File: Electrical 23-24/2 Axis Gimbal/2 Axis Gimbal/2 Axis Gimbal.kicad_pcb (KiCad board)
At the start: 2 copper layers, 24.2 x 38.5 mm, 28 parts, among them IC1 BNO085, IC2 AP1086DL-13, J1 Conn_01x06_Socket, J2 Conn_01x06_Socket, U1 ATtiny404-SS

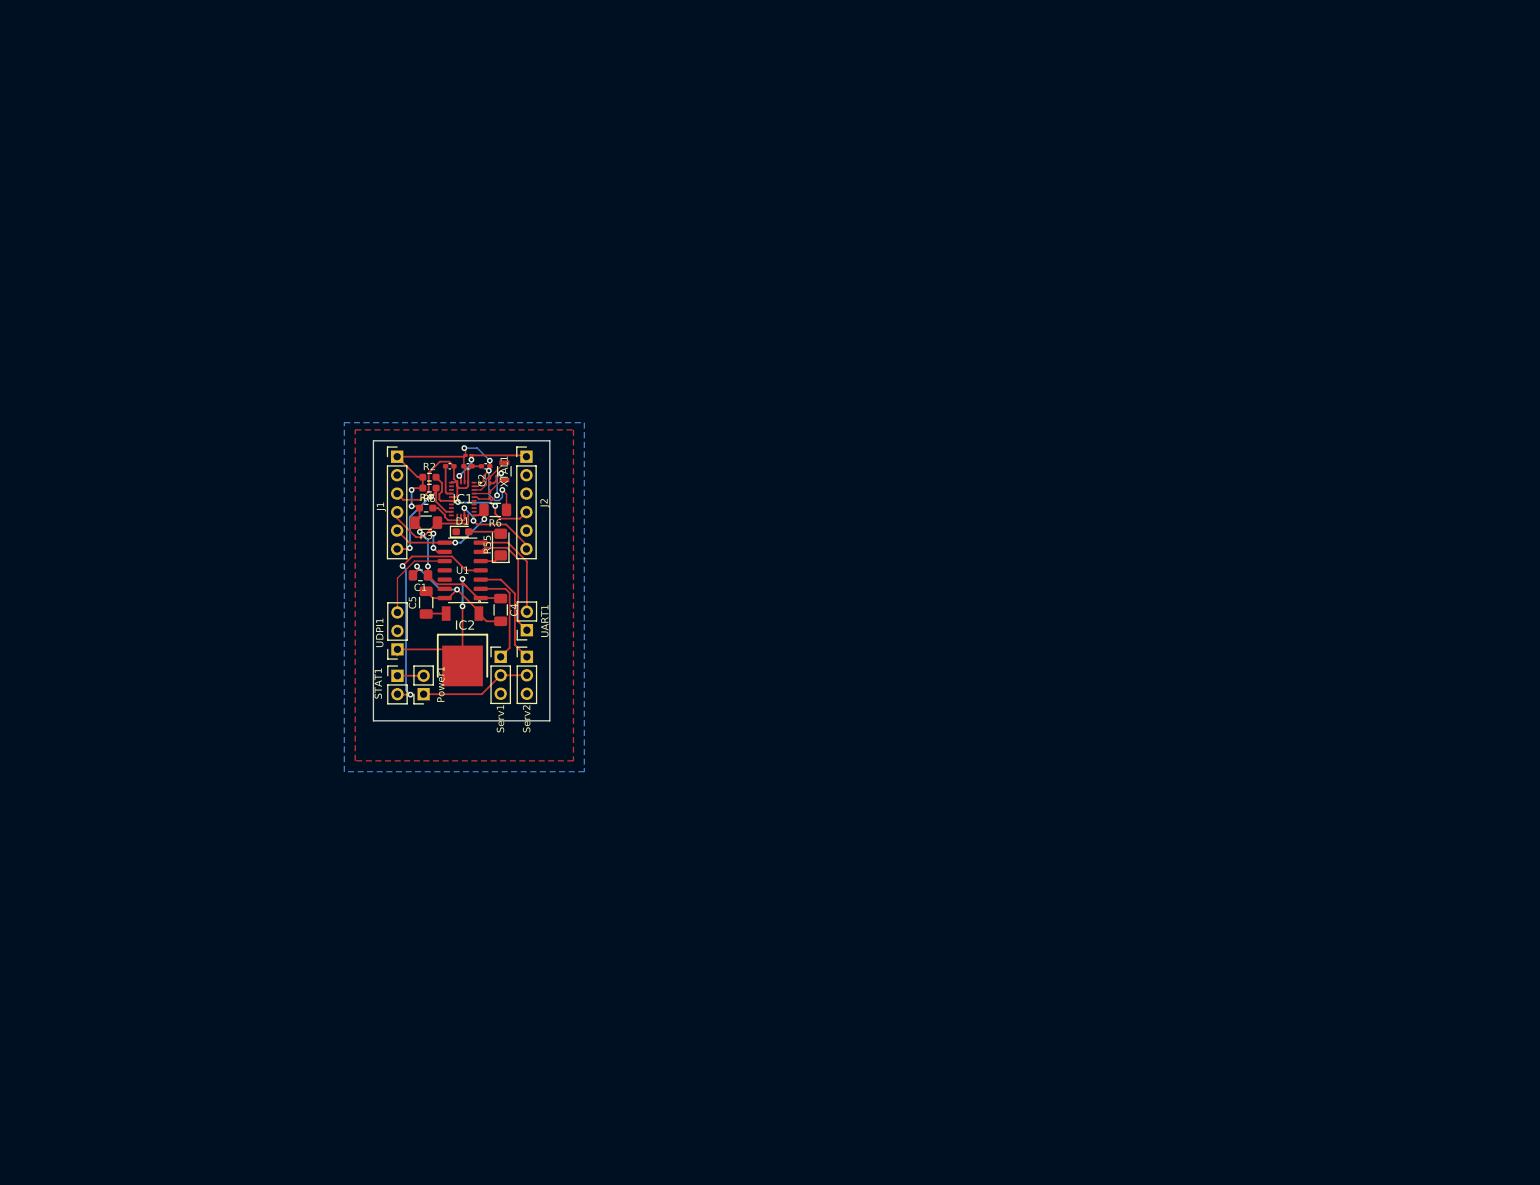
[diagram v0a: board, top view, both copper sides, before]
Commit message: Finished Gimbal Board
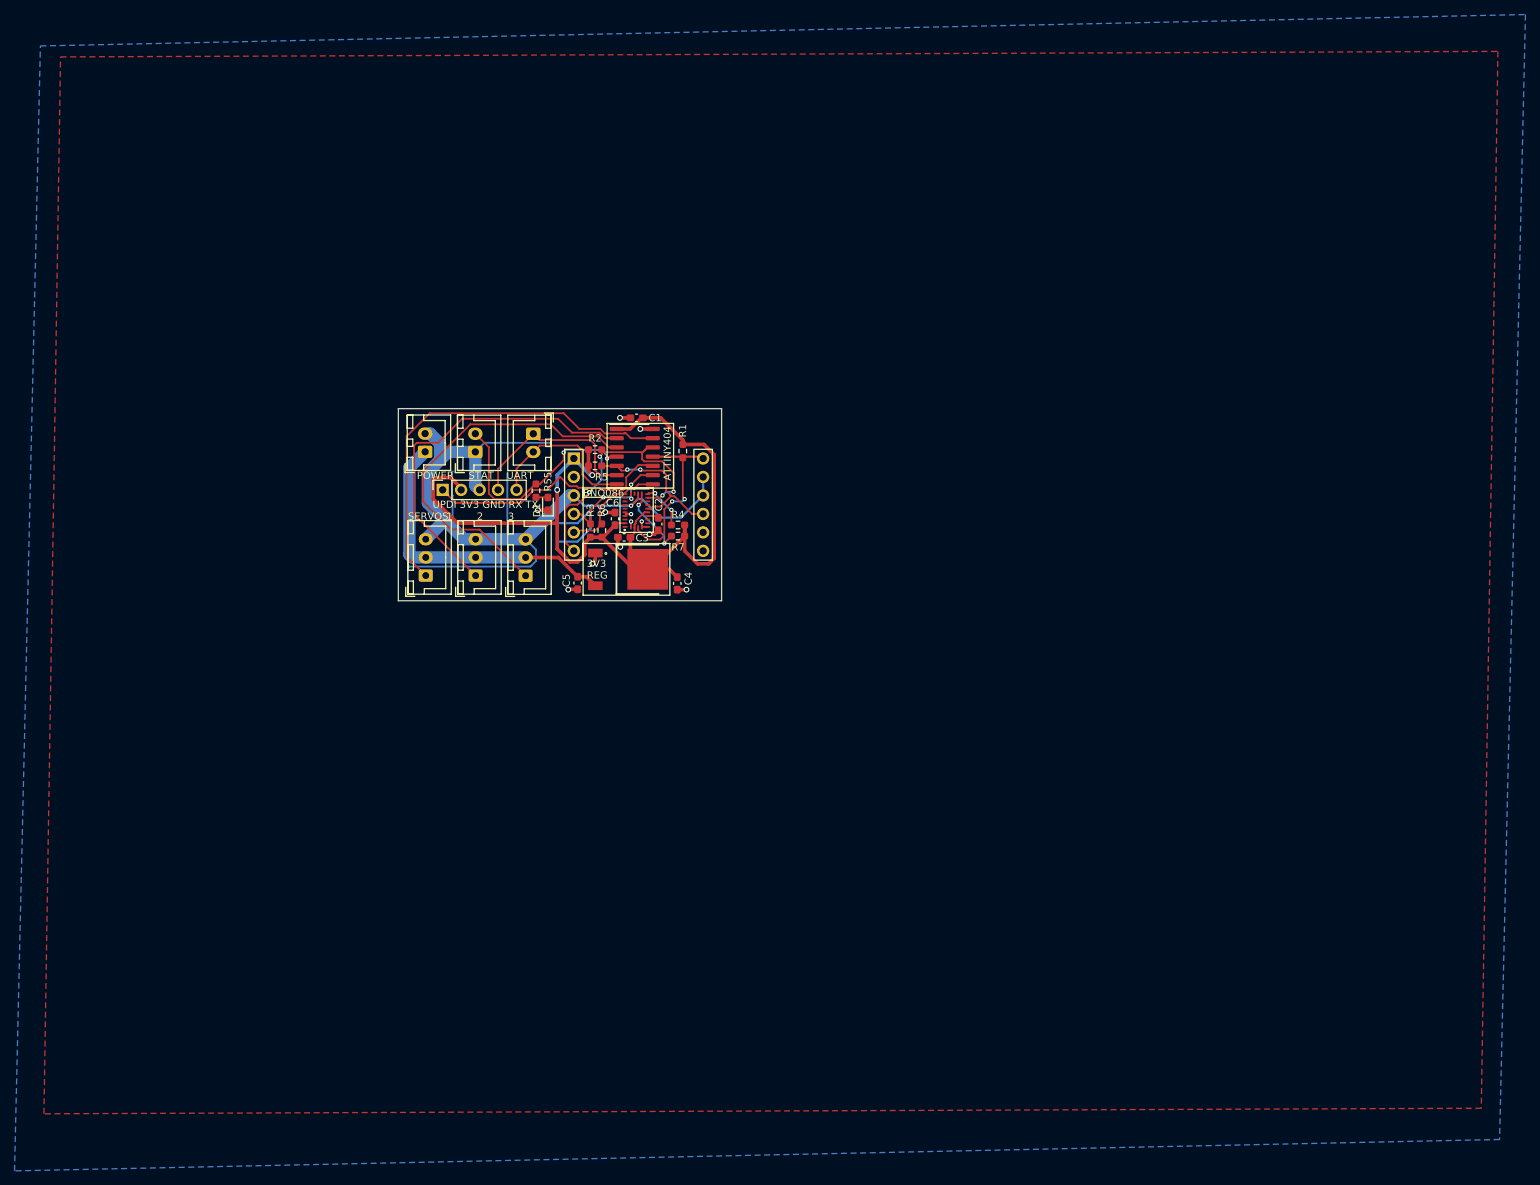
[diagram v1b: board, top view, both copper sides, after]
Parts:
- removed the C2 at (87.0, 77.9)
- removed the C3 at (87.0, 79.9)
- removed J1, J2: Conn_01x06_Socket, Connector_PinHeader_2.54mm:PinHeader_1x06_P2.54mm_Vertical
- removed XTAL1: ABS07-32.768KHZ-7-T, 32Crys:XTAL_ABS07-32.768KHZ-7-T_ABR
- added G***: LOGO, LOGO, B.Cu at (108.1, 81.3)
- added R7: 2.2k, Resistor_SMD:R_0603_1608Metric_Pad0.98x0.95mm_HandSolder, F.Cu at (112.9, 85.6)
- added Servo3: Conn_01x03_Pin, Connector_JST:JST_XH_B3B-XH-A_1x03_P2.50mm_Vertical, F.Cu at (91.9, 91.0)
- added U2: ~, gimbal:breakout, F.Cu at (107.4, 81.3)
- C1: value C_10uF -> 10u; footprint Capacitor_SMD:C_0805_2012Metric_Pad1.18x1.45mm_HandSolder -> Capacitor_SMD:C_0603_1608Metric_Pad1.08x0.95mm_HandSolder
- C2: renamed from D-CUP2; value C_0.1uF -> 0.1u; footprint Capacitor_SMD:C_0402_1005Metric_Pad0.74x0.62mm_HandSolder -> Capacitor_SMD:C_0603_1608Metric_Pad1.08x0.95mm_HandSolder
- C3: renamed from D-CUP3; value C_0.1uF -> 0.1u; footprint Capacitor_SMD:C_0402_1005Metric_Pad0.74x0.62mm_HandSolder -> Capacitor_SMD:C_0603_1608Metric_Pad1.08x0.95mm_HandSolder
- C4, C5: value C_100uF -> 10u; footprint Capacitor_SMD:C_1206_3216Metric_Pad1.33x1.80mm_HandSolder -> Capacitor_SMD:C_0603_1608Metric_Pad1.08x0.95mm_HandSolder
- C6: renamed from D-CUP1; value C_0.1uF -> 0.1u; footprint Capacitor_SMD:C_0402_1005Metric_Pad0.74x0.62mm_HandSolder -> Capacitor_SMD:C_0603_1608Metric_Pad1.08x0.95mm_HandSolder
- IC1: footprint BNO085:BNO085 -> gimbal:BNO085
- IC2: footprint VReg3.3:TO252-3L_1 -> gimbal:TO252-3L_1
- Power1, UART1: footprint Connector_PinSocket_2.54mm:PinSocket_1x02_P2.54mm_Vertical -> Connector_JST:JST_XH_B2B-XH-A_1x02_P2.50mm_Vertical
- R1: value 10KR -> 10k; footprint Resistor_SMD:R_0201_0603Metric_Pad0.64x0.40mm_HandSolder -> Resistor_SMD:R_0603_1608Metric_Pad0.98x0.95mm_HandSolder
- R2, R5: value 10KR -> 10k
- R3, R6: footprint Resistor_SMD:R_1206_3216Metric_Pad1.30x1.75mm_HandSolder -> Resistor_SMD:R_0603_1608Metric_Pad0.98x0.95mm_HandSolder
- R4: value 10KR -> 2.2k
- R55: value RES -> 140; footprint LED_SMD:LED_1206_3216Metric_Pad1.42x1.75mm_HandSolder -> Resistor_SMD:R_0603_1608Metric_Pad0.98x0.95mm_HandSolder
- STAT1: footprint Connector_PinHeader_2.54mm:PinHeader_1x02_P2.54mm_Vertical -> Connector_JST:JST_XH_B2B-XH-A_1x02_P2.50mm_Vertical
- Servo1: renamed from Serv1; footprint Connector_PinHeader_2.54mm:PinHeader_1x03_P2.54mm_Vertical -> Connector_JST:JST_XH_B3B-XH-A_1x03_P2.50mm_Vertical
- Servo2: renamed from Serv2; footprint Connector_PinHeader_2.54mm:PinHeader_1x03_P2.54mm_Vertical -> Connector_JST:JST_XH_B3B-XH-A_1x03_P2.50mm_Vertical
- UDPI1: footprint Connector_PinSocket_2.54mm:PinSocket_1x03_P2.54mm_Vertical -> Connector_PinSocket_2.54mm:PinSocket_1x05_P2.54mm_Vertical
- moved C1 36.8 mm to (107.2, 69.3)
- moved R4 34.7 mm to (112.9, 84.1)
- moved Power1 33.3 mm to (78.1, 74.0), turned to 90 degrees
- moved STAT1 32.6 mm to (85.0, 74.0), turned to 90 degrees
- moved IC2 30.7 mm to (110.2, 90.2), turned to -90 degrees
- moved C2 29.7 mm to (110.2, 83.9), turned to 90 degrees
- moved R1 29.5 mm to (113.5, 73.9), turned to -90 degrees
- moved U1 28.4 mm to (106.9, 74.7), turned to 0 degrees
- moved UART1 27.0 mm to (93.0, 71.5), turned to -90 degrees
- moved C4 24.5 mm to (112.8, 92.1)
- moved IC1 23.9 mm to (107.1, 82.1), turned to 180 degrees
- moved C3 23.6 mm to (105.5, 85.8), turned to 180 degrees
- moved R5 23.4 mm to (101.5, 73.7)
- moved R2 22.8 mm to (101.5, 75.9)
- moved UDPI1 22.8 mm to (80.5, 79.2), turned to 90 degrees
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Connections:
- C5 pad 1: +5V -> +BATT
- IC1 pad 10: GND -> 3.3
- IC1 pad 15: unconnected-(IC1-ENV_SCL_-Pad15) -> Net-(IC1-ENV_SCL_)
- IC1 pad 16: unconnected-(IC1-ENV_SDA-Pad16) -> Net-(IC1-ENV_SDA)
- IC1 pad 17: unconnected-(IC1-SA0/H_MOSI_-Pad17) -> GND
- IC1 pad 18: CSN -> unconnected-(IC1-H_CSN-Pad18)
- IC1 pad 26: Net-(IC1-XOUT32/CLKSEL1) -> GND
- IC1 pad 27: Net-(IC1-XIN32) -> unconnected-(IC1-XIN32-Pad27)
- IC2 pad 2: +5V -> +BATT
- R4 pad 1: 3.3 -> Net-(IC1-ENV_SCL_)
- R4 pad 2: CSN -> 3.3
- R55 pad 1: LED -> STAT
- U1 pad 11: unconnected-(U1-PA1-Pad11) -> BOOTN
- U1 pad 12: unconnected-(U1-PA2-Pad12) -> INT
- U1 pad 13: unconnected-(U1-PA3-Pad13) -> PWM 1
- U1 pad 2: PWM 1 -> PWM 2
- U1 pad 3: PWM 2 -> PWM 3
- U1 pad 5: LED -> RST
- UDPI1 pad 1: 3.3 -> UPDI
- UDPI1 pad 2: GND -> 3.3
- UDPI1 pad 3: UPDI -> GND
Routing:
- net GND: track 59.4 -> 156.2 mm, vias 4 -> 13
- net PWM 3: track 0.00 -> 53.1 mm
- net PWM 1: track 13.5 -> 56.9 mm
- net 3.3: track 89.4 -> 130.9 mm, vias 10 -> 2
- net PWM 2: track 14.9 -> 51.9 mm
- net +BATT: track 15.3 -> 42.4 mm
- net INT: track 16.1 -> 38.3 mm, vias 2 -> 4
- net UPDI: track 12.2 -> 34.1 mm
- net CSN: track 18.4 -> 0.00 mm, vias 2 -> 0
- net BOOTN: track 12.1 -> 24.7 mm
- net Net-(IC1-ENV_SDA): track 0.00 -> 9.91 mm, vias 0 -> 2
- net RX: track 16.3 -> 25.6 mm
- net TX: track 14.3 -> 22.2 mm
- net Net-(IC1-ENV_SCL_): track 0.00 -> 6.44 mm, vias 0 -> 2
- net Net-(IC1-XIN32): track 6.15 -> 0.00 mm
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- added copper zone on F.Cu, net GND
- removed copper zone on F.Cu, net (none)
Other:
- board size 24.2 x 38.5 mm -> 44.5 x 26.4 mm
- board text added: "1"
- board text added: "2"
- board text added: "3"
- board text added: "3V3"
- board text added: "3V3 REG"
- board text added: "3VO"
- board text added: "ATTINY404"
- board text added: "Anthony Cheung Ari Bobesh"
- board text added: "BNO086"
- board text added: "BOOT"
- board text added: "CS"
- board text added: "DI"
- board text added: "GND"
- board text added: "Gimbal Board V1 04/02/24"
- board text added: "INT"
- board text added: "P0"
- board text added: "P1"
- board text added: "POWER"
- board text added: "PWM"
- board text added: "RST"
- board text added: "RX"
- board text added: "SCL"
- board text added: "SDA"
- board text added: "SERVOS"
- board text added: "STAT"
- board text added: "TX"
- board text added: "UART"
- board text added: "UPDI 3V3 GND RX TX"
- board text added: "VBAT"
